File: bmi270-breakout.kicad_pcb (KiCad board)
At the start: 2 copper layers, 15.2 x 20.6 mm, 16 parts, among them CN1 AFC10-S04QCA-00, CN2 AFC10-S04QCA-00, J1 Conn_01x06_Pin, J2 Conn_01x04_Pin, U1 BMI270

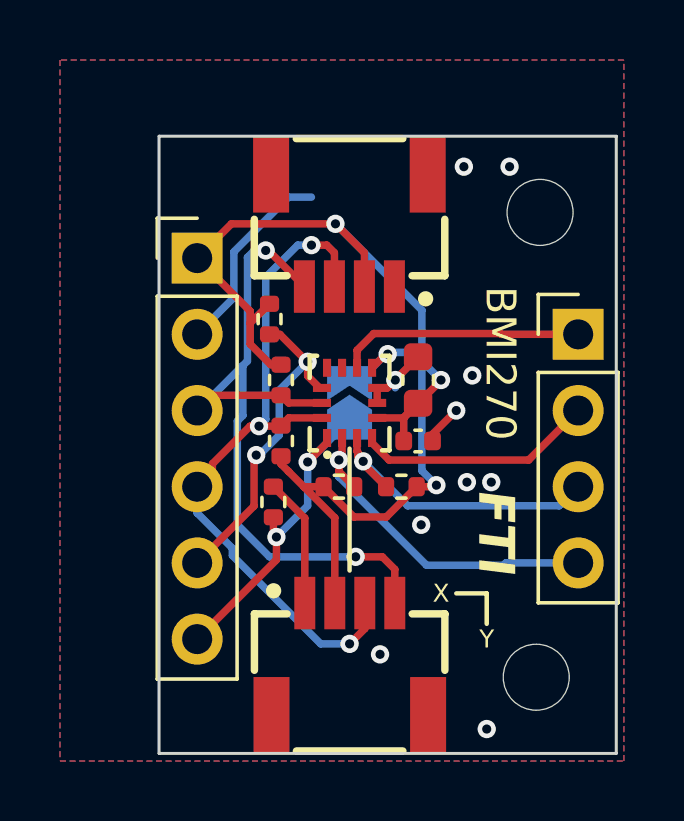
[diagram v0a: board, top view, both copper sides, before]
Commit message: allign mounting holes
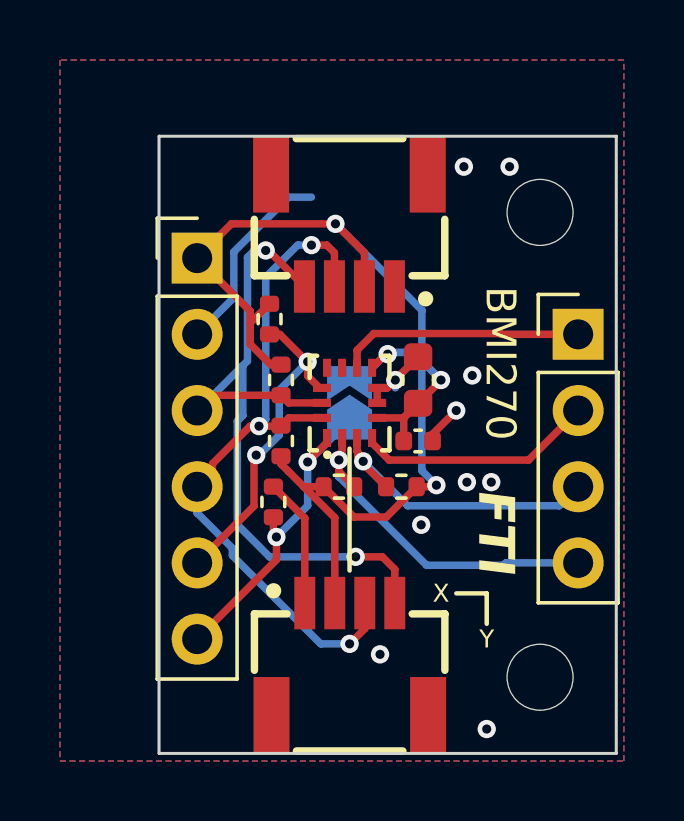
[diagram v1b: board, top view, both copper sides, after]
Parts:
- moved H2 0.13 mm to (158.8, 110.5)
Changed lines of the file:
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@@
 	(footprint "MountingHole:MountingHole_2.2mm_M2"
 		(layer "F.Cu")
-		(at 158.623 110.49)
+		(at 158.75 110.49)
 		(descr "Mounting Hole 2.2mm, no annular, M2")
 		(tags "mounting hole 2.2mm no annular m2")
